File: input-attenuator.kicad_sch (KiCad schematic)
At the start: 85 parts, among them J1 DC_INTF, J2 DC_INTF, J3 RX_1_RF, J4 RX_2_RF, J5 RF_IN, K1 EE2-5TNU-L, K2 EE2-5TNU-L, K3 EE2-5TNU-L, K4 EE2-5TNU-L, Q1 BC858, Q10 MMBT3904, Q2 BC858, Q3 MMBT3904, Q4 BC858, Q5 BC858, Q6 BC858, Q7 BC858, Q8 BC858, Q9 BC858, U1 74HC00, U2 74HC00, U3 74HC00, U4 74HC00, U5 74HC00, U6 74HC595, U7 TPS7A4501DCQT, U8 LP339

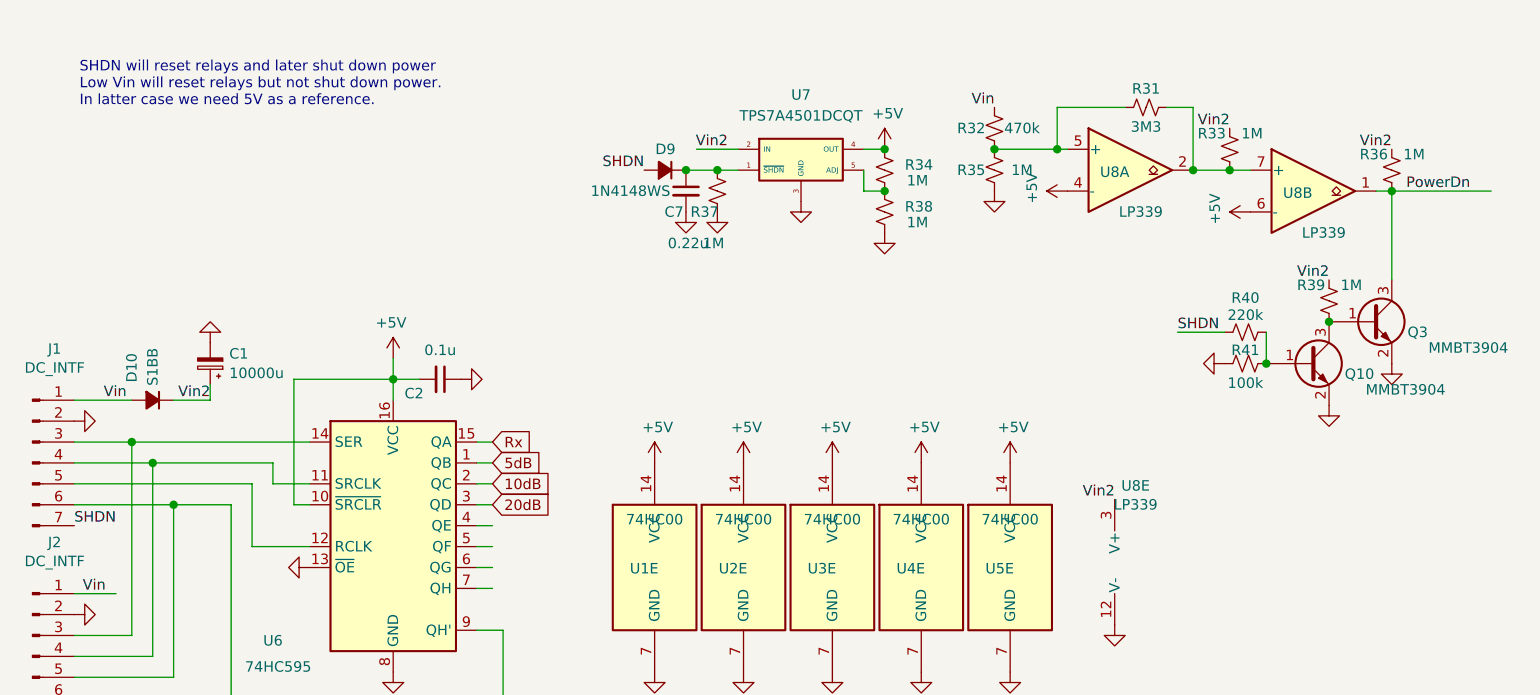
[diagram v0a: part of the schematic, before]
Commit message: final
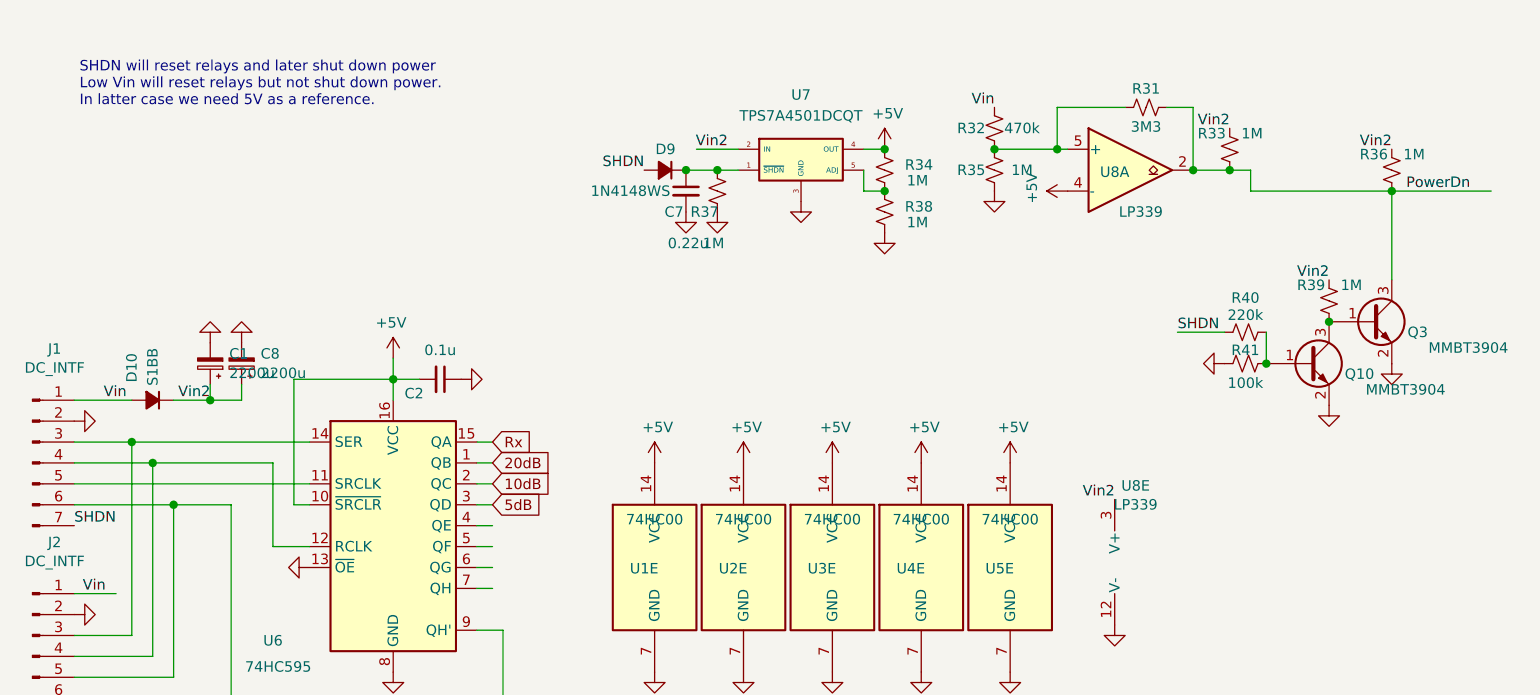
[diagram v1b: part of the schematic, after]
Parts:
- removed unit 2 of U8
- added C8: 2200u, Capacitor_THT:CP_Radial_D12.5mm_P7.50mm, symbol Device:CP_Small
- C1: value 10000u -> 2200u; footprint Capacitor_SMD:CP_Elec_6.3x5.4_Nichicon -> Capacitor_THT:CP_Radial_D12.5mm_P7.50mm
- U6: footprint Package_SO:SO-16_5.3x10.2mm_P1.27mm -> Package_SO:SO-16_3.9x9.9mm_P1.27mm
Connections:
- net 20dB: now also U6.1 (QB); no longer U6.3 (QD)
- net 5dB: now also U6.3 (QD); no longer U6.1 (QB)
- net GND: now also C8.2
- net PowerDn: now also R31.1, R33.1, U8.2
- net Vin2: now also C8.1
- net at J1.4 (Pin_4), J2.4 (Pin_4): now also U6.12 (RCLK); no longer U6.11 (SRCLK)
- net at J1.5 (Pin_5): now also U6.11 (SRCLK); no longer U6.12 (RCLK)
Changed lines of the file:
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@@
   (junction (at 29.845 160.02) (diameter 1.016) (color 0 0 0 0))
   (junction (at 32.385 165.1) (diameter 1.016) (color 0 0 0 0))
+  (junction (at 36.83 152.4) (diameter 1.016) (color 0 0 0 0))
   (junction (at 38.1 40.005) (diameter 1.016) (color 0 0 0 0))
   (junction (at 38.1 57.15) (diameter 1.016) (color 0 0 0 0))
@@
     (stroke (width 0) (type solid) (color 0 0 0 0))
   )
-  (wire (pts (xy 20.32 162.56) (xy 41.91 162.56))
+  (wire (pts (xy 20.32 162.56) (xy 48.895 162.56))
     (stroke (width 0) (type solid) (color 0 0 0 0))
   )
@@
     (stroke (width 0) (type solid) (color 0 0 0 0))
   )
+  (wire (pts (xy 36.83 152.4) (xy 40.64 152.4))
+    (stroke (width 0) (type solid) (color 0 0 0 0))
+  )
   (wire (pts (xy 38.1 38.1) (xy 38.1 40.005))
     (stroke (width 0) (type solid) (color 0 0 0 0))
@@
     (stroke (width 0) (type solid) (color 0 0 0 0))
   )
-  (wire (pts (xy 41.91 85.09) (xy 46.99 85.09))
-    (stroke (width 0) (type solid) (color 0 0 0 0))
-  )
-  (wire (pts (xy 41.91 90.805) (xy 41.91 85.09))
+  (wire (pts (xy 40.64 152.4) (xy 40.64 150.495))
     (stroke (width 0) (type solid) (color 0 0 0 0))
   )
-  (wire (pts (xy 41.91 162.56) (xy 41.91 170.18))
+  (wire (pts (xy 41.91 85.09) (xy 46.99 85.09))
     (stroke (width 0) (type solid) (color 0 0 0 0))
   )
-  (wire (pts (xy 41.91 170.18) (xy 48.895 170.18))
+  (wire (pts (xy 41.91 90.805) (xy 41.91 85.09))
     (stroke (width 0) (type solid) (color 0 0 0 0))
   )
-  (wire (pts (xy 44.45 160.02) (xy 44.45 162.56))
+  (wire (pts (xy 44.45 160.02) (xy 44.45 170.18))
     (stroke (width 0) (type solid) (color 0 0 0 0))
   )
-  (wire (pts (xy 44.45 162.56) (xy 48.895 162.56))
+  (wire (pts (xy 44.45 170.18) (xy 48.895 170.18))
     (stroke (width 0) (type solid) (color 0 0 0 0))
   )
@@
     (stroke (width 0) (type solid) (color 0 0 0 0))
   )
+  (wire (pts (xy 163.195 127) (xy 163.195 124.46))
+    (stroke (width 0) (type solid) (color 0 0 0 0))
+  )
+  (wire (pts (xy 163.195 127) (xy 180.34 127))
+    (stroke (width 0) (type solid) (color 0 0 0 0))
+  )
   (wire (pts (xy 165.1 38.1) (xy 165.1 40.005))
     (stroke (width 0) (type solid) (color 0 0 0 0))
@@
     (stroke (width 0) (type solid) (color 0 0 0 0))
   )
-  (wire (pts (xy 178.435 127) (xy 180.34 127))
-    (stroke (width 0) (type solid) (color 0 0 0 0))
-  )
   (wire (pts (xy 180.34 127) (xy 180.34 137.795))
     (stroke (width 0) (type solid) (color 0 0 0 0))
@@
     )
   )
-  (global_label "5dB" (shape input) (at 71.12 160.02 0)
+  (global_label "20dB" (shape input) (at 71.12 160.02 0)
     (effects (font (size 1.27 1.27)) (justify left))
-    (property "Intersheet References" "${INTERSHEET_REFS}" (id 0) (at 78.6857 159.9406 0)
+    (property "Intersheet References" "${INTERSHEET_REFS}" (id 0) (at 79.8952 159.9406 0)
       (effects (font (size 1.27 1.27)) (justify left) hide)
     )
@@
     )
   )
-  (global_label "20dB" (shape input) (at 71.12 165.1 0)
+  (global_label "5dB" (shape input) (at 71.12 165.1 0)
     (effects (font (size 1.27 1.27)) (justify left))
-    (property "Intersheet References" "${INTERSHEET_REFS}" (id 0) (at 79.8952 165.0206 0)
+    (property "Intersheet References" "${INTERSHEET_REFS}" (id 0) (at 78.6857 165.0206 0)
       (effects (font (size 1.27 1.27)) (justify left) hide)
     )
@@
     (pin "1")
   )
-  (symbol (lib_id "power:+5V") (at 163.195 129.54 90) (unit 1)
-    (in_bom yes) (on_board yes)
-    (property "Reference" "#PWR0148" (id 0) (at 167.005 129.54 0)
-      (effects (font (size 1.27 1.27)) hide)
-    )
-    (property "Value" "+5V" (id 1) (at 158.8706 129.1717 0))
-    (property "Footprint" "" (id 2) (at 163.195 129.54 0)
-      (effects (font (size 1.27 1.27)) hide)
-    )
-    (property "Datasheet" "" (id 3) (at 163.195 129.54 0)
-      (effects (font (size 1.27 1.27)) hide)
-    )
-    (pin "1")
-  )
   (symbol (lib_id "power:+5V") (at 165.1 71.12 180) (unit 1)
     (in_bom yes) (on_board yes)
@@
     (pin "1")
   )
+  (symbol (lib_id "power:GND") (at 40.64 145.415 180) (unit 1)
+    (in_bom yes) (on_board yes)
+    (property "Reference" "#PWR0153" (id 0) (at 40.64 139.065 0)
+      (effects (font (size 1.27 1.27)) hide)
+    )
+    (property "Value" "GND" (id 1) (at 40.513 140.9192 0)
+      (effects (font (size 1.27 1.27)) hide)
+    )
+    (property "Footprint" "" (id 2) (at 40.64 145.415 0)
+      (effects (font (size 1.27 1.27)) hide)
+    )
+    (property "Datasheet" "" (id 3) (at 40.64 145.415 0)
+      (effects (font (size 1.27 1.27)) hide)
+    )
+    (pin "1")
+  )
   (symbol (lib_id "power:GND") (at 41.91 95.885 270) (unit 1)
     (in_bom yes) (on_board yes)
@@
       (effects (font (size 1.27 1.27)) (justify right))
     )
-    (property "Value" "10000u" (id 1) (at 39.1414 149.1234 0)
+    (property "Value" "2200u" (id 1) (at 39.141 149.123 0)
       (effects (font (size 1.27 1.27)) (justify right))
     )
-    (property "Footprint" "Capacitor_SMD:CP_Elec_6.3x5.4_Nichicon" (id 2) (at 36.83 147.955 0)
+    (property "Footprint" "Capacitor_THT:CP_Radial_D12.5mm_P7.50mm" (id 2) (at 36.83 147.955 0)
       (effects (font (size 1.27 1.27)) hide)
     )
@@
     (pin "2")
   )
+  (symbol (lib_id "Device:CP_Small") (at 40.64 147.955 180) (unit 1)
+    (in_bom yes) (on_board yes)
+    (property "Reference" "C8" (id 0) (at 42.9514 146.7612 0)
+      (effects (font (size 1.27 1.27)) (justify right))
+    )
+    (property "Value" "2200u" (id 1) (at 42.951 149.123 0)
+      (effects (font (size 1.27 1.27)) (justify right))
+    )
+    (property "Footprint" "Capacitor_THT:CP_Radial_D12.5mm_P7.50mm" (id 2) (at 40.64 147.955 0)
+      (effects (font (size 1.27 1.27)) hide)
+    )
+    (property "Datasheet" "~" (id 3) (at 40.64 147.955 0)
+      (effects (font (size 1.27 1.27)) hide)
+    )
+    (pin "1")
+    (pin "2")
+  )
   (symbol (lib_id "Device:C_Small") (at 44.45 95.885 270) (unit 1)
     (in_bom yes) (on_board yes)
@@
     (pin "5")
   )
-  (symbol (lib_id "Comparator:LM339") (at 170.815 127 0) (unit 2)
-    (in_bom yes) (on_board yes)
-    (property "Reference" "U8" (id 0) (at 168.91 127.235 0))
-    (property "Value" "LP339" (id 1) (at 172.085 132.074 0))
-    (property "Footprint" "Package_SO:SO-14_3.9x8.65mm_P1.27mm" (id 2) (at 169.545 124.46 0)
-      (effects (font (size 1.27 1.27)) hide)
-    )
-    (property "Datasheet" "https://www.st.com/resource/en/datasheet/lm139.pdf" (id 3) (at 172.085 121.92 0)
-      (effects (font (size 1.27 1.27)) hide)
-    )
-    (pin "1")
-    (pin "6")
-    (pin "7")
-  )
   (symbol (lib_id "74xx:74HC00") (at 90.805 172.72 0) (unit 5)
     (in_bom yes) (on_board yes)
@@
     (property "Reference" "U6" (id 0) (at 44.45 181.61 0))
     (property "Value" "74HC595" (id 1) (at 45.085 184.785 0))
-    (property "Footprint" "Package_SO:SO-16_5.3x10.2mm_P1.27mm" (id 2) (at 59.055 167.64 0)
+    (property "Footprint" "Package_SO:SO-16_3.9x9.9mm_P1.27mm" (id 2) (at 59.055 167.64 0)
       (effects (font (size 1.27 1.27)) hide)
     )
@@
       (reference "#PWR0147") (unit 1) (value "GND") (footprint "")
     )
-    (path "/580483ba-39e3-4efc-8eeb-6522e33be8e8"
-      (reference "#PWR0148") (unit 1) (value "+5V") (footprint "")
-    )
     (path "/c947ab05-4742-494e-b7fe-632a05628c8f"
       (reference "#PWR0149") (unit 1) (value "GND") (footprint "")
@@
       (reference "#PWR0152") (unit 1) (value "GND") (footprint "")
     )
+    (path "/3e44b944-75b2-458b-a4b6-319ed679d7aa"
+      (reference "#PWR0153") (unit 1) (value "GND") (footprint "")
+    )
     (path "/00000000-0000-0000-0000-00005f2f2f18"
-      (reference "C1") (unit 1) (value "10000u") (footprint "Capacitor_SMD:CP_Elec_6.3x5.4_Nichicon")
+      (reference "C1") (unit 1) (value "2200u") (footprint "Capacitor_THT:CP_Radial_D12.5mm_P7.50mm")
     )
     (path "/00000000-0000-0000-0000-00005f2ebfc9"
@@
       (reference "C7") (unit 1) (value "0.22u") (footprint "Capacitor_SMD:C_0805_2012Metric")
     )
+    (path "/7699ad8e-2776-4a76-aa81-f71fb3040c25"
+      (reference "C8") (unit 1) (value "2200u") (footprint "Capacitor_THT:CP_Radial_D12.5mm_P7.50mm")
+    )
     (path "/00000000-0000-0000-0000-00005f1e54e1"
       (reference "D1") (unit 1) (value "1N4148WS") (footprint "Diode_SMD:D_SOD-323")
@@
     )
     (path "/00000000-0000-0000-0000-00005f259000"
-      (reference "U6") (unit 1) (value "74HC595") (footprint "Package_SO:SO-16_5.3x10.2mm_P1.27mm")
+      (reference "U6") (unit 1) (value "74HC595") (footprint "Package_SO:SO-16_3.9x9.9mm_P1.27mm")
     )
     (path "/8354ecd4-2a4f-44f8-a737-ff9cdb5f7927"
@@
       (reference "U8") (unit 1) (value "LP339") (footprint "Package_SO:SO-14_3.9x8.65mm_P1.27mm")
     )
-    (path "/83430977-3e55-4b8c-bc38-a585c8d1731b"
-      (reference "U8") (unit 2) (value "LP339") (footprint "Package_SO:SO-14_3.9x8.65mm_P1.27mm")
-    )
     (path "/b903cbde-9215-48dd-89f9-54d7dabe3bb1"
